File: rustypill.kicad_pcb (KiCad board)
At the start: 2 copper layers, 69 x 48 mm, 50 parts, among them IC1 DS3231, J1 USB, J2 PROG, J3 GPIOB, J4 GPIOA, J5 LCD1602, J6 IDC_10P, J7 I2C, M2 MountingHole_2.7mm_M2.5, M3 MountingHole_2.7mm_M2.5, M4 MountingHole_2.7mm_M2.5, SW1 Reset, U1 AMS1117-3.3, U2 AT24C512C-SSHD-T, U3 ESP-12F, U4 STM32F103C8Tx, Y1 8MHz

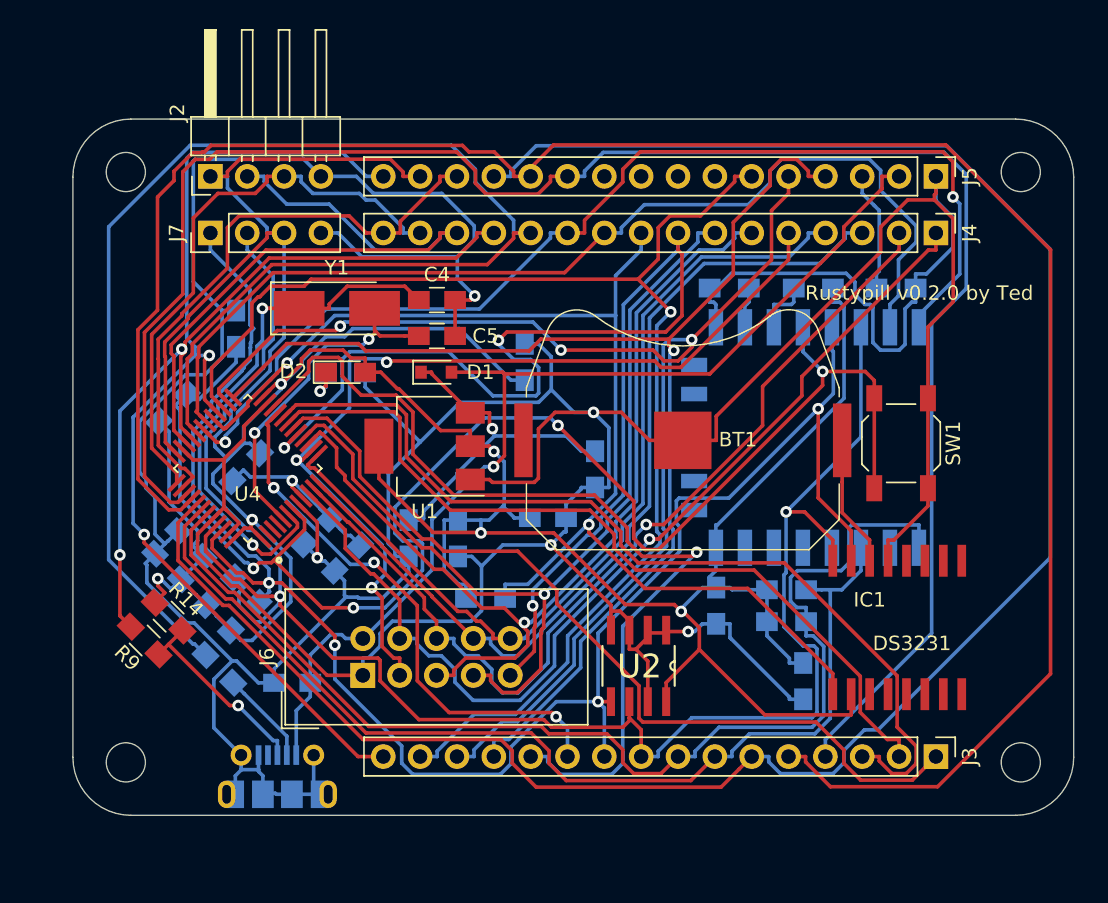
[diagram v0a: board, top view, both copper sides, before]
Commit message: ...
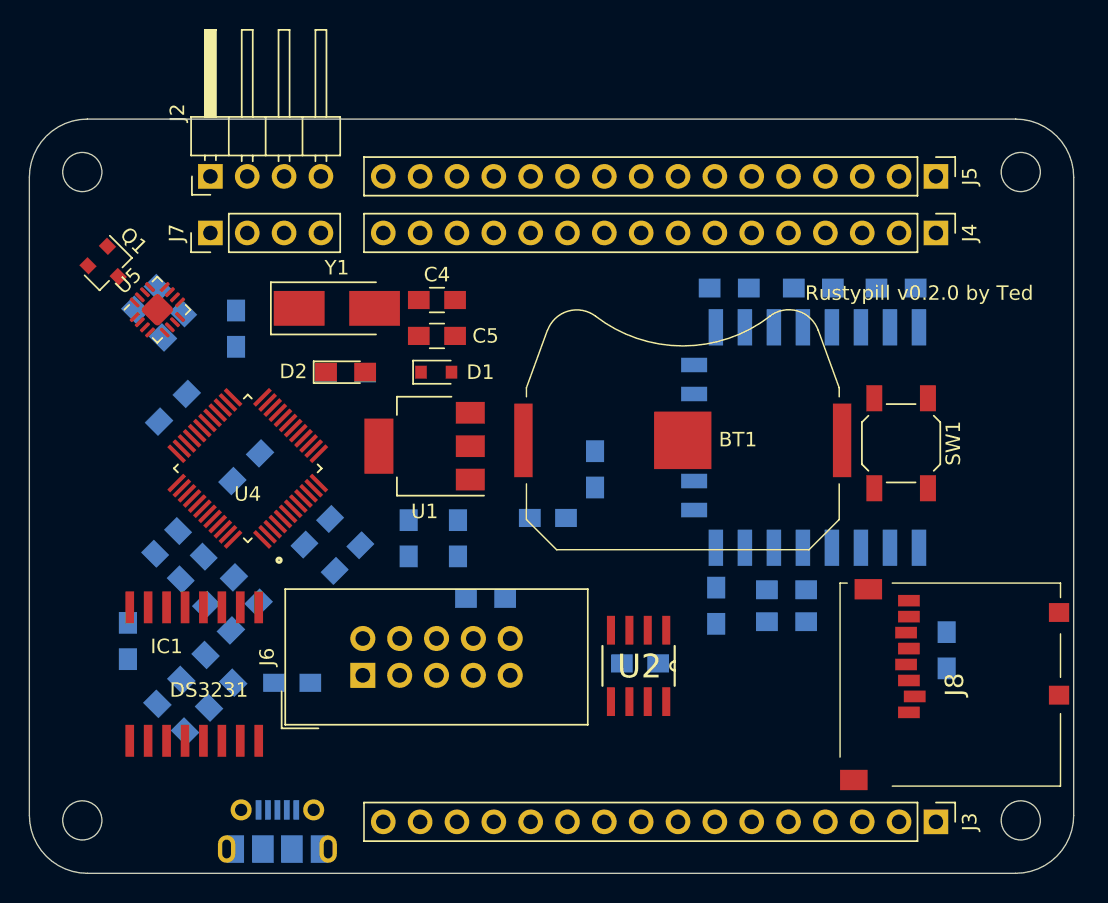
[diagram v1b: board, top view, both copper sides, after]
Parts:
- added C16: 100nF, Capacitors_SMD:C_0805_HandSoldering, B.Cu at (74.6, 104.5)
- added C17: 100nF, Capacitors_SMD:C_0805_HandSoldering, B.Cu at (128.1, 128.6)
- added J8: Micro_SD_Card, lib:473340001, F.Cu at (128.6, 131.0)
- added Q1: BC548, TO_SOT_Packages_SMD:SOT-23, F.Cu at (70.3, 102.2)
- added R15: Rbl, Resistors_SMD:R_0805_HandSoldering, B.Cu at (73.1, 106.1)
- added U5: PCF8574, lib:VQFN-16-1EP_3x3mm_P0.5mm_EP1.68x1.68mm, F.Cu at (73.7, 105.1)
- R14, R9: moved to B.Cu
- moved IC1 48.6 mm to (76.2, 130.3)
- moved C11 46.6 mm to (71.6, 128.0), turned to 90 degrees
- moved C12 22.2 mm to (107.0, 129.5), turned to 180 degrees
- moved R14 6.97 mm to (74.6, 133.3)
- moved R9 5.06 mm to (76.3, 131.6)
- moved M3 5.00 mm to (68.5, 140.3)
- moved J3 4.50 mm to (127.3, 140.4)
- moved M4 4.00 mm to (133.2, 140.3)
- moved J1 3.78 mm to (82.0, 142.0)
- moved  M1 3.00 mm to (68.5, 95.7)
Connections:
- J5 pad 11: B3 -> LCD_D4
- J5 pad 12: B4 -> LCD_D5
- J5 pad 13: B5 -> LCD_D6
- J5 pad 14: A15 -> LCD_D7
- J5 pad 16: B15 -> LCD_BL
- J5 pad 4: B12 -> LCD_RS
- J5 pad 5: B13 -> LCD_RW
- J5 pad 6: B14 -> LCD_EN
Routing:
- net GND: track 378.6 -> 0.00 mm, vias 5 -> 0
- net +3V3: track 259.3 -> 0.00 mm, vias 6 -> 0
- net B4: track 145.5 -> 0.00 mm
- net B5: track 143.5 -> 0.00 mm
- net B3: track 128.7 -> 0.00 mm
- net B8: track 128.0 -> 0.00 mm, vias 2 -> 0
- net B9: track 122.2 -> 0.00 mm, vias 4 -> 0
- net IC_RST: track 103.3 -> 0.00 mm, vias 4 -> 0
- net A11: track 100.6 -> 0.00 mm
- net B14: track 91.8 -> 0.00 mm, vias 1 -> 0
- net B13: track 89.6 -> 0.00 mm, vias 3 -> 0
- net B12: track 86.3 -> 0.00 mm, vias 1 -> 0
- net A7: track 84.6 -> 0.00 mm, vias 3 -> 0
- net 32KHZ_IN: track 84.4 -> 0.00 mm, vias 2 -> 0
- net B7: track 80.0 -> 0.00 mm
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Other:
- board size 69 x 48 mm -> 72 x 52 mm

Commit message: ...
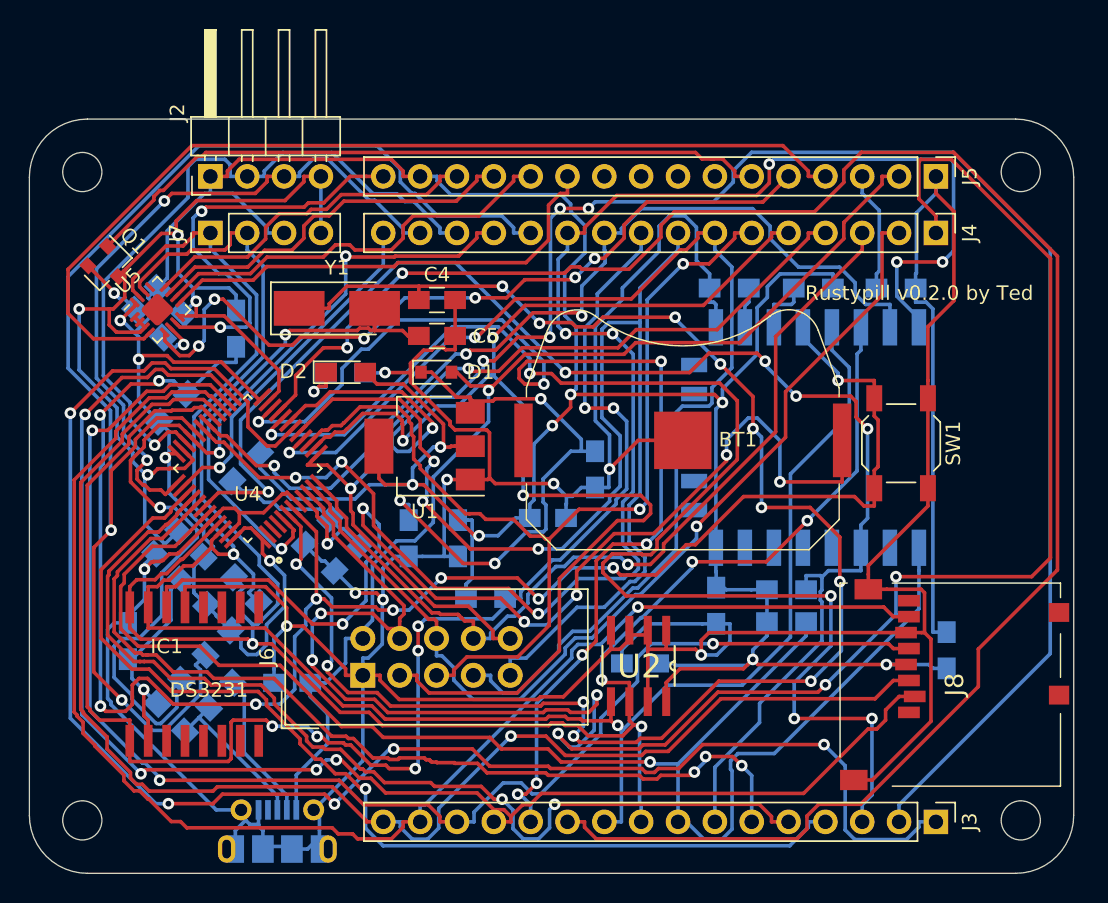
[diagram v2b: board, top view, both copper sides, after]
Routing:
- net GND: track 0.00 -> 415.1 mm, vias 0 -> 13
- net +3V3: track 0.00 -> 267.0 mm, vias 0 -> 13
- net B8: track 0.00 -> 143.9 mm, vias 0 -> 5
- net B9: track 0.00 -> 133.0 mm, vias 0 -> 2
- net B10: track 0.00 -> 132.7 mm, vias 0 -> 2
- net A0: track 0.00 -> 130.0 mm, vias 0 -> 6
- net IC_RST: track 0.00 -> 123.0 mm, vias 0 -> 10
- net B1: track 0.00 -> 122.0 mm, vias 0 -> 5
- net Net-(C4-Pad1): track 0.00 -> 114.1 mm, vias 0 -> 12
- net B0: track 0.00 -> 113.4 mm, vias 0 -> 5
- net A10: track 0.00 -> 112.3 mm, vias 0 -> 8
- net 32KHZ_IN: track 0.00 -> 107.5 mm, vias 0 -> 7
- net B7: track 0.00 -> 102.1 mm, vias 0 -> 1
- net B6: track 0.00 -> 100.1 mm, vias 0 -> 5
- net B12: track 0.00 -> 99.6 mm, vias 0 -> 4
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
